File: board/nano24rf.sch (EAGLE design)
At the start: 2 parts

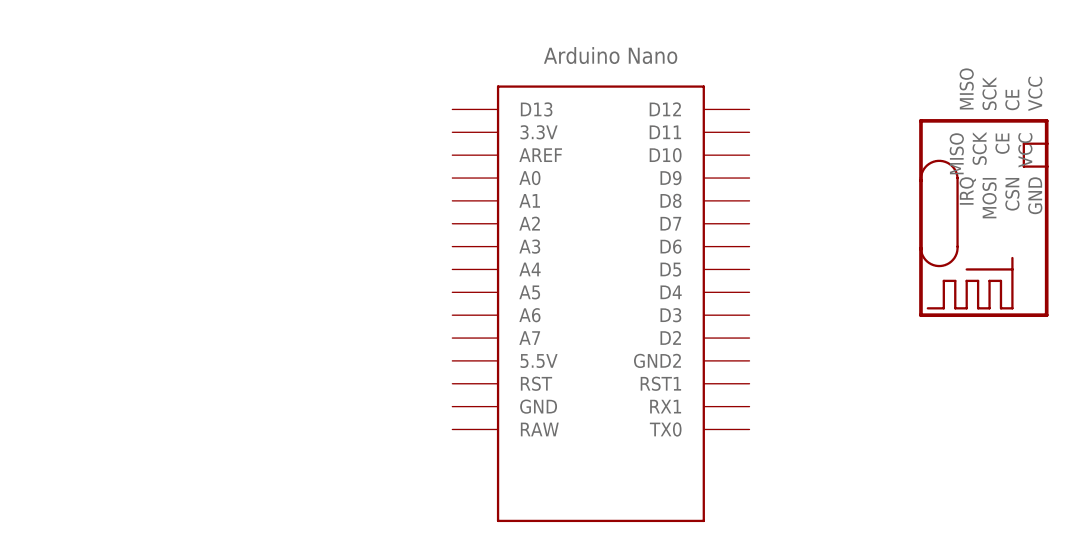
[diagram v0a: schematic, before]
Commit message: with mini for lols
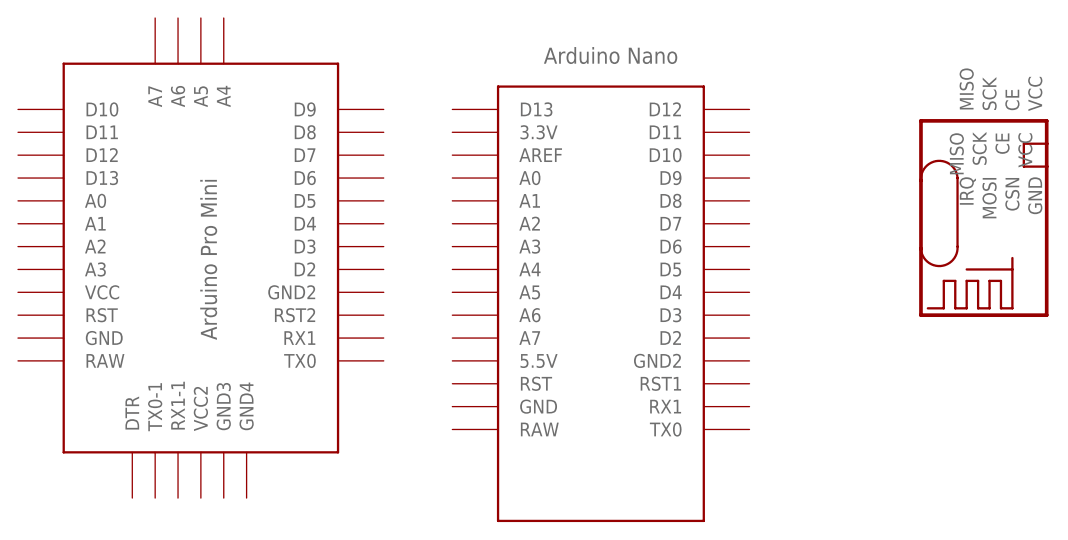
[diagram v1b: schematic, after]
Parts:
- added U$3: PRO-MINI, Arduino-clone:PRO-MINI
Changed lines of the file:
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@@
 <part name="U$1" library="Arduino-clone" deviceset="NANO" device=""/>
 <part name="U$2" library="Arduino-clone" deviceset="NRF24" device=""/>
+<part name="U$3" library="Arduino-clone" deviceset="PRO-MINI" device=""/>
 </parts>
 <sheets>
@@
 <instance part="U$1" gate="G$1" x="60.96" y="50.8"/>
 <instance part="U$2" gate="G$1" x="95.25" y="60.96"/>
+<instance part="U$3" gate="G$1" x="7.62" y="58.42" rot="R180"/>
 </instances>
 <busses>
